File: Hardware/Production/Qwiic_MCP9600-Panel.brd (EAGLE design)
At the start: 22.9 x 39.4 mm, 43 parts, among them J1 PTH, U16 MCP9600-SMD

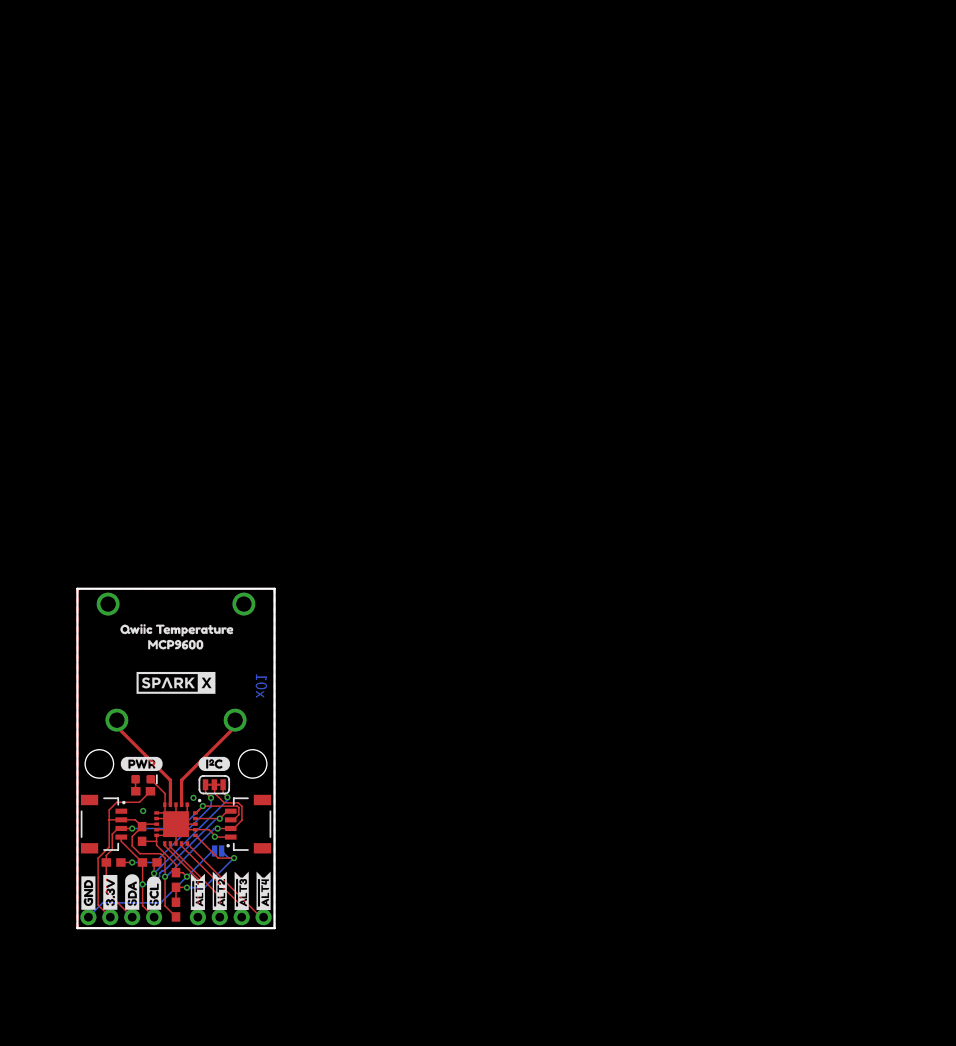
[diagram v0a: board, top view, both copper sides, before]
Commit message: Added production files
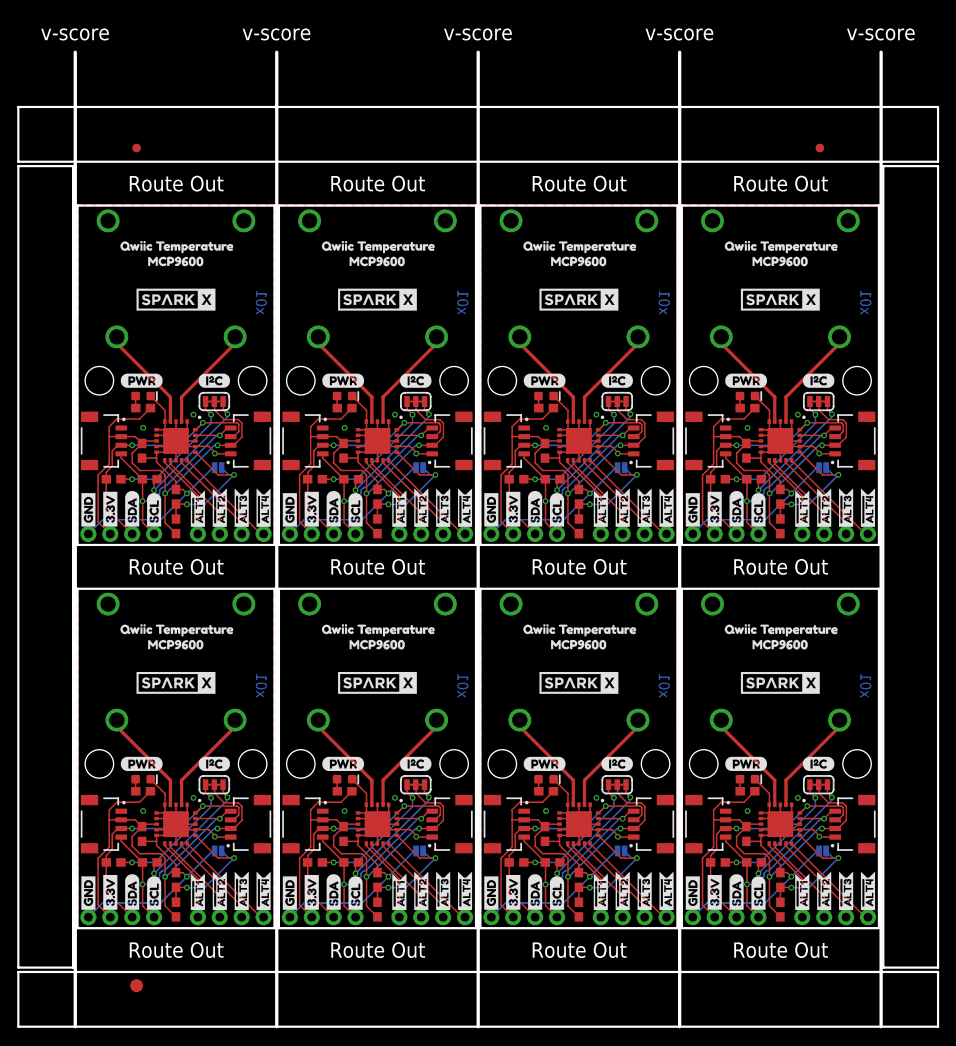
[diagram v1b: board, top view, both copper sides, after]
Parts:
- removed FRAME1: FRAME-LETTER, SparkFun-Aesthetics:CREATIVE_COMMONS
- added C2, C3, C4, C5, C6, C7, C8: 0.1uF, SparkFun-Capacitors:0603
- added D2, D3, D4, D5, D6, D7, D8: RED, SparkFun-LED:LED-0603
- added E$1, E$2: (no value), SparkFun-Aesthetics:FIDUCIAL-1X2
- added E$3: (no value), SparkFun-Retired:FIDUCIAL-1.5X3
- added I2C1, I2C2, I2C3, I2C4, I2C5, I2C6, I2C7: (no value), SparkFun-Jumpers:SMT-JUMPER_3_2-NC_TRACE_SILK
- added J10, J11, J14, J15, J18, J19, J22, J23, J26, J27, J30, J31, J6, J7: (no value), SparkFun-Connectors:JST04_1MM_RA
- added J12, J16, J20, J24, J28, J32, J8: (no value), SparkFun-Connectors:1X04_NO_SILK
- added J13, J17, J21, J25, J29, J5, J9: PTH, SparkX:1X04_NO_SILK
- added JP10, JP11, JP14, JP15, JP18, JP19, JP22, JP23, JP26, JP27, JP30, JP31, JP4, JP5: STAND-OFF, SparkFun:STAND-OFF
- added JP12, JP16, JP20, JP24, JP28, JP32, JP6: PCB_THERMOCOUPLE, MCP9600:PCC-SMP
- added JP13, JP17, JP21, JP25, JP29, JP3, JP7: (no value), SparkFun-Jumpers:SMT-JUMPER_2_NO_SILK
- added LOGO2, LOGO3, LOGO4, LOGO5, LOGO6, LOGO7, LOGO8: OSHW-LOGOMINI, SparkFun-Aesthetics:OSHW-LOGO-MINI
- added R10, R15, R20, R25, R30, R35, R40: 10k, SparkFun-Resistors:0603
- added R11, R16, R21, R26, R31, R36, R6: 1k, SparkFun-Resistors:0603
- added R12, R17, R22, R27, R32, R37, R7: 43k, SparkFun-Resistors:0603
- added R13, R14, R18, R19, R23, R24, R28, R29, R33, R34, R38, R39, R8, R9: 2.2k, SparkFun-Resistors:0603
- added U$100, U$107, U$124, U$131, U$148, U$155, U$172, U$179, U$28, U$35, U$52, U$59, U$76, U$83: (no value), Labels:SCL-[)
- added U$101, U$125, U$149, U$173, U$29, U$53, U$77: (no value), Labels:PWR-()-04
- added U$102, U$126, U$150, U$174, U$30, U$54, U$78: (no value), Labels:I_SUPER2_C-()-04
- added U$103, U$104, U$127, U$128, U$151, U$152, U$175, U$176, U$31, U$32, U$55, U$56, U$79, U$80: (no value), Labels:3.3V
- added U$105, U$106, U$129, U$130, U$153, U$154, U$177, U$178, U$33, U$34, U$57, U$58, U$81, U$82: (no value), Labels:GND-04
- added U$108, U$109, U$132, U$133, U$156, U$157, U$180, U$181, U$36, U$37, U$60, U$61, U$84, U$85: (no value), Labels:SDA-[)
- added U$110, U$134, U$158, U$182, U$38, U$62, U$86: (no value), SparkFun-Aesthetics:QWIIC_5.5MM
- added U$111, U$135, U$159, U$183, U$39, U$63, U$87: (no value), MCP9600:MCP96000
- added U$112, U$136, U$160, U$184, U$40, U$64, U$88: (no value), MCP9600:ADR_#_0X600
- added U$113, U$117, U$137, U$141, U$161, U$165, U$185, U$189, U$41, U$45, U$65, U$69, U$89, U$93: (no value), MCP9600:#ALT10
- added U$114, U$118, U$138, U$142, U$162, U$166, U$186, U$190, U$42, U$46, U$66, U$70, U$90, U$94: (no value), MCP9600:#ALT20
- added U$115, U$119, U$139, U$143, U$163, U$167, U$187, U$191, U$43, U$47, U$67, U$71, U$91, U$95: (no value), MCP9600:#ALT30
- added U$116, U$120, U$140, U$144, U$164, U$168, U$188, U$192, U$44, U$48, U$68, U$72, U$92, U$96: (no value), MCP9600:#ALT40
- added U$121, U$145, U$16, U$169, U$49, U$73, U$97: (no value), buzzard_labels (2):QWIIC_TEMPERATURE2
- added U$122, U$123, U$146, U$147, U$170, U$171, U$24, U$26, U$50, U$51, U$74, U$75, U$98, U$99: (no value), SparkX:SPARKX-MEDIUM
- added U1, U2, U3, U4, U5, U6, U7: MCP9600-SMD, MCP9600:MQFN-20
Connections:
- new net !ALT10: J12.3, U2.14
- new net !ALT11: J12.4, U2.15
- new net !ALT12: J12.2, U2.12
- new net !ALT13: J16.1, U3.11
- new net !ALT14: J16.3, U3.14
- new net !ALT15: J16.4, U3.15
- new net !ALT16: J16.2, U3.12
- new net !ALT17: J20.1, U4.11
- new net !ALT18: J20.3, U4.14
- new net !ALT19: J20.4, U4.15
- new net !ALT20: J20.2, U4.12
- new net !ALT21: J24.1, U5.11
- new net !ALT22: J24.3, U5.14
- new net !ALT23: J24.4, U5.15
- new net !ALT24: J24.2, U5.12
- new net !ALT25: J28.1, U6.11
- new net !ALT26: J28.3, U6.14
- new net !ALT27: J28.4, U6.15
- new net !ALT28: J28.2, U6.12
- new net !ALT29: J32.1, U7.11
- new net !ALT30: J32.3, U7.14
- new net !ALT31: J32.4, U7.15
- new net !ALT32: J32.2, U7.12
- new net !ALT5: J8.1, U1.11
- new net !ALT6: J8.3, U1.14
- new net !ALT7: J8.4, U1.15
- new net !ALT8: J8.2, U1.12
- new net !ALT9: J12.1, U2.11
- new net 3.3V1: C2.1, I2C1.2, J5.2, J6.2, J7.2, R10.2, R6.1, U1.8
- new net 3.3V2: C3.1, I2C2.2, J10.2, J11.2, J9.2, R11.1, R15.2, U2.8
- new net 3.3V3: C4.1, I2C3.2, J13.2, J14.2, J15.2, R16.1, R20.2, U3.8
- new net 3.3V4: C5.1, I2C4.2, J17.2, J18.2, J19.2, R21.1, R25.2, U4.8
- new net 3.3V5: C6.1, I2C5.2, J21.2, J22.2, J23.2, R26.1, R30.2, U5.8
- new net 3.3V6: C7.1, I2C6.2, J25.2, J26.2, J27.2, R31.1, R35.2, U6.8
- new net 3.3V7: C8.1, I2C7.2, J29.2, J30.2, J31.2, R36.1, R40.2, U7.8
- new net ADDR1: JP3.1, R10.1, R7.1, U1.16
- new net ADDR2: JP7.1, R12.1, R15.1, U2.16
- new net ADDR3: JP13.1, R17.1, R20.1, U3.16
- new net ADDR4: JP17.1, R22.1, R25.1, U4.16
- new net ADDR5: JP21.1, R27.1, R30.1, U5.16
- new net ADDR6: JP25.1, R32.1, R35.1, U6.16
- new net ADDR7: JP29.1, R37.1, R40.1, U7.16
- new net GND1: C2.2, D2.C, J5.1, J6.1, J7.1, JP3.2, R7.2, U1.1, U1.10, U1.13, U1.17, U1.18, U1.21, U1.3, U1.5, U1.6, U1.7, U1.9
- new net GND2: C3.2, D3.C, J10.1, J11.1, J9.1, JP7.2, R12.2, U2.1, U2.10, U2.13, U2.17, U2.18, U2.21, U2.3, U2.5, U2.6, U2.7, U2.9
- new net GND3: C4.2, D4.C, J13.1, J14.1, J15.1, JP13.2, R17.2, U3.1, U3.10, U3.13, U3.17, U3.18, U3.21, U3.3, U3.5, U3.6, U3.7, U3.9
- new net GND4: C5.2, D5.C, J17.1, J18.1, J19.1, JP17.2, R22.2, U4.1, U4.10, U4.13, U4.17, U4.18, U4.21, U4.3, U4.5, U4.6, U4.7, U4.9
- new net GND5: C6.2, D6.C, J21.1, J22.1, J23.1, JP21.2, R27.2, U5.1, U5.10, U5.13, U5.17, U5.18, U5.21, U5.3, U5.5, U5.6, U5.7, U5.9
- new net GND6: C7.2, D7.C, J25.1, J26.1, J27.1, JP25.2, R32.2, U6.1, U6.10, U6.13, U6.17, U6.18, U6.21, U6.3, U6.5, U6.6, U6.7, U6.9
- new net GND7: C8.2, D8.C, J29.1, J30.1, J31.1, JP29.2, R37.2, U7.1, U7.10, U7.13, U7.17, U7.18, U7.21, U7.3, U7.5, U7.6, U7.7, U7.9
- new net N$10: JP6.-, U1.4
- new net N$11: D3.A, R11.2
- new net N$12: I2C2.1, R14.2
- new net N$13: I2C2.3, R13.2
- new net N$14: JP12.+, U2.2
- new net N$15: JP12.-, U2.4
- new net N$16: D4.A, R16.2
- new net N$17: I2C3.1, R19.2
- new net N$18: I2C3.3, R18.2
- new net N$19: JP16.+, U3.2
- new net N$20: JP16.-, U3.4
- new net N$21: D5.A, R21.2
- new net N$22: I2C4.1, R24.2
- new net N$23: I2C4.3, R23.2
- new net N$24: JP20.+, U4.2
- new net N$25: JP20.-, U4.4
- new net N$26: D6.A, R26.2
- new net N$27: I2C5.1, R29.2
- new net N$28: I2C5.3, R28.2
- new net N$29: JP24.+, U5.2
- new net N$30: JP24.-, U5.4
- new net N$31: D7.A, R31.2
- new net N$32: I2C6.1, R34.2
- new net N$33: I2C6.3, R33.2
- new net N$34: JP28.+, U6.2
- new net N$35: JP28.-, U6.4
- new net N$36: D8.A, R36.2
- new net N$37: I2C7.1, R39.2
- new net N$38: I2C7.3, R38.2
- new net N$39: JP32.+, U7.2
- new net N$40: JP32.-, U7.4
- new net N$6: D2.A, R6.2
- new net N$7: I2C1.1, R9.2
- new net N$8: I2C1.3, R8.2
- new net N$9: JP6.+, U1.2
- new net SCL1: J5.4, J6.4, J7.4, R9.1, U1.19
- new net SCL2: J10.4, J11.4, J9.4, R14.1, U2.19
- new net SCL3: J13.4, J14.4, J15.4, R19.1, U3.19
- new net SCL4: J17.4, J18.4, J19.4, R24.1, U4.19
- new net SCL5: J21.4, J22.4, J23.4, R29.1, U5.19
- new net SCL6: J25.4, J26.4, J27.4, R34.1, U6.19
- new net SCL7: J29.4, J30.4, J31.4, R39.1, U7.19
- new net SDA1: J5.3, J6.3, J7.3, R8.1, U1.20
- new net SDA2: J10.3, J11.3, J9.3, R13.1, U2.20
- new net SDA3: J13.3, J14.3, J15.3, R18.1, U3.20
- new net SDA4: J17.3, J18.3, J19.3, R23.1, U4.20
- new net SDA5: J21.3, J22.3, J23.3, R28.1, U5.20
- new net SDA6: J25.3, J26.3, J27.3, R33.1, U6.20
- new net SDA7: J29.3, J30.3, J31.3, R38.1, U7.20
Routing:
- net 3.3V5: track 0.00 -> 57.7 mm, vias 0 -> 2
- net 3.3V7: track 0.00 -> 57.7 mm, vias 0 -> 2
- net 3.3V4: track 0.00 -> 57.7 mm, vias 0 -> 2
- net 3.3V6: track 0.00 -> 57.7 mm, vias 0 -> 2
- net 3.3V1: track 0.00 -> 57.7 mm, vias 0 -> 2
- net 3.3V3: track 0.00 -> 57.7 mm, vias 0 -> 2
- net 3.3V2: track 0.00 -> 57.7 mm, vias 0 -> 2
- net GND6: track 0.00 -> 54.6 mm, vias 0 -> 4
- net GND5: track 0.00 -> 54.6 mm, vias 0 -> 4
- net GND4: track 0.00 -> 54.6 mm, vias 0 -> 4
- net GND2: track 0.00 -> 54.6 mm, vias 0 -> 4
- net GND7: track 0.00 -> 54.6 mm, vias 0 -> 4
- net GND1: track 0.00 -> 54.6 mm, vias 0 -> 4
- net GND3: track 0.00 -> 54.6 mm, vias 0 -> 4
- net SDA6: track 0.00 -> 30.5 mm, vias 0 -> 2
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- added copper zone on layer 1, net GND1
- added copper zone on layer 16, net GND1
- added copper zone on layer 1, net GND2
- added copper zone on layer 16, net GND2
- added copper zone on layer 1, net GND3
- added copper zone on layer 16, net GND3
- added copper zone on layer 1, net GND4
- added copper zone on layer 16, net GND4
- added copper zone on layer 1, net GND5
- added copper zone on layer 16, net GND5
- added copper zone on layer 1, net GND6
- added copper zone on layer 16, net GND6
- added copper zone on layer 1, net GND7
- added copper zone on layer 16, net GND7
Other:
- board size 22.9 x 39.4 mm -> 106.7 x 113 mm
- board text added: "Route Out"
- board text added: "v-score"
- board text removed: "Fischer Moseley"
